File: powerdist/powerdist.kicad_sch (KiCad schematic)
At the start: 61 parts, among them J1 Conn_01x02_Socket, J10 Conn_01x02_Pin, J11 Conn_01x02_Pin, J12 Conn_01x02_Pin, J13 Conn_01x02_Pin, J2 Conn_01x02_Socket, J3 Conn_01x04_Socket, J4 Conn_01x04_Pin, J5 Conn_01x02_Socket, J6 Conn_01x02_Socket, J7 Conn_01x02_Socket, J8 Conn_01x02_Socket, J9 Conn_01x04_Socket, Q1 SI4178DY, Q2 SI4178DY, Q3 SI4178DY, Q4 SI4178DY, Q5 DMN2056U, Q6 DMN2056U, Q7 DMN2056U, Q8 DMN2056U

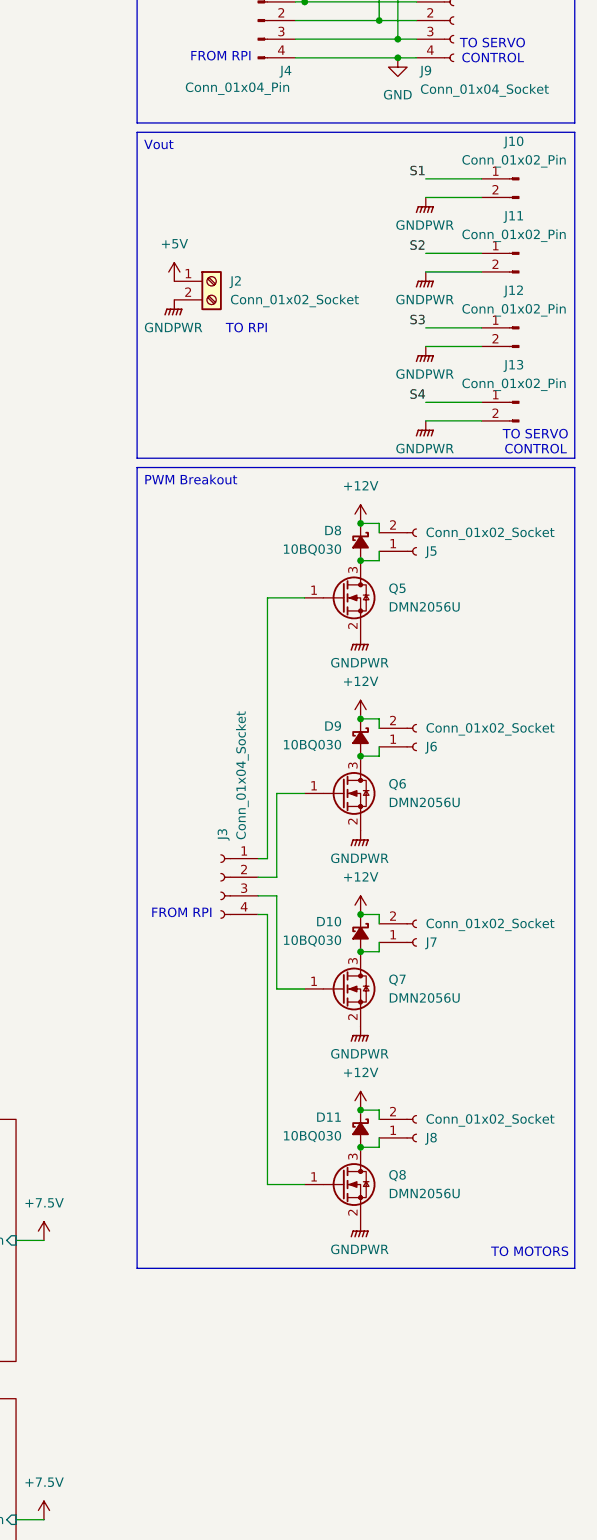
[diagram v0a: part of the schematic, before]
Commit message: local 29/10
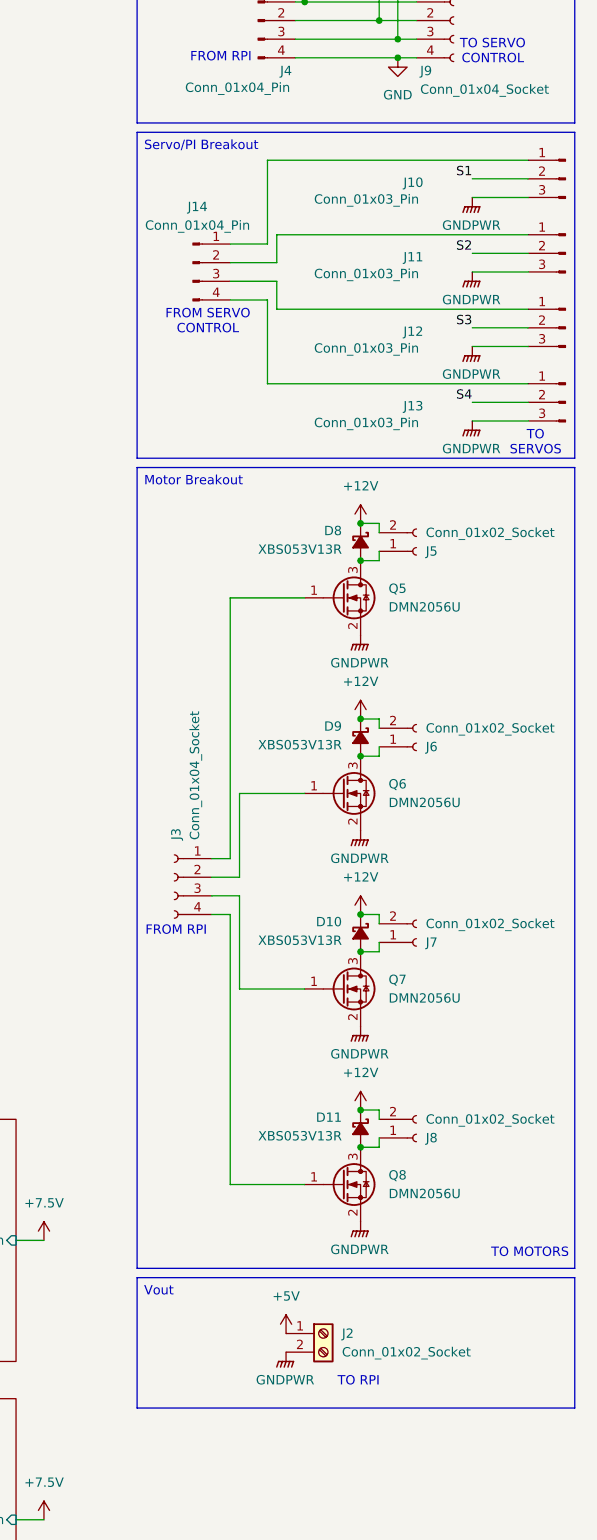
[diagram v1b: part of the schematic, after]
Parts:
- added J14: Conn_01x04_Pin, Connector_PinHeader_2.54mm:PinHeader_1x04_P2.54mm_Vertical, symbol Connector:Conn_01x04_Pin
- D10, D11, D8, D9: value 10BQ030 -> XBS053V13R; footprint Diode_SMD:D_SMB -> Diode_SMD:D_SOD-323_HandSoldering
- J10, J11, J12, J13: value Conn_01x02_Pin -> Conn_01x03_Pin; footprint Connector_PinHeader_2.54mm:PinHeader_1x02_P2.54mm_Vertical -> Connector_PinHeader_2.54mm:PinHeader_1x03_P2.54mm_Vertical; symbol Connector:Conn_01x02_Pin -> Connector:Conn_01x03_Pin
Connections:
- net GND: now also J10.3 (Pin_3), J11.3 (Pin_3), J12.3 (Pin_3), J13.3 (Pin_3); no longer J10.2 (Pin_2), J11.2 (Pin_2), J12.2 (Pin_2), J13.2 (Pin_2)
- net S1: now also J10.2 (Pin_2); no longer J10.1 (Pin_1)
- net S2: now also J11.2 (Pin_2); no longer J11.1 (Pin_1)
- net S3: now also J12.2 (Pin_2); no longer J12.1 (Pin_1)
- net S4: now also J13.2 (Pin_2); no longer J13.1 (Pin_1)
- new net: J10.1 (Pin_1), J14.1 (Pin_1)
- new net: J13.1 (Pin_1), J14.4 (Pin_4)
- new net: J12.1 (Pin_1), J14.3 (Pin_3)
- new net: J11.1 (Pin_1), J14.2 (Pin_2)
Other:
- note added: "FROM SERVO CONTROL"
- note added: "TO SERVOS"
- moved on the sheet: J2, J3
